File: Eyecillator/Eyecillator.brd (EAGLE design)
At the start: 92.4 x 35.5 mm, 24 parts, among them IC1 4093, IC2 LM567

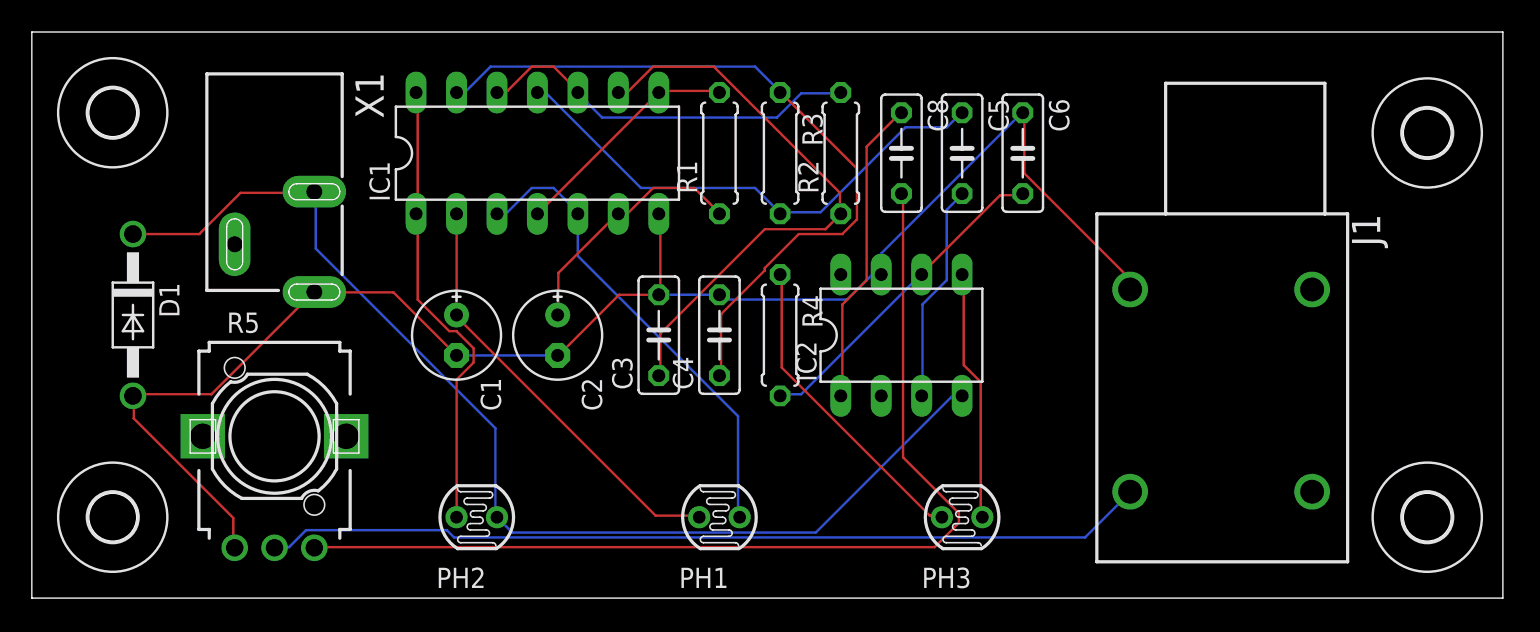
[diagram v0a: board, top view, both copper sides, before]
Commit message: Add files via upload
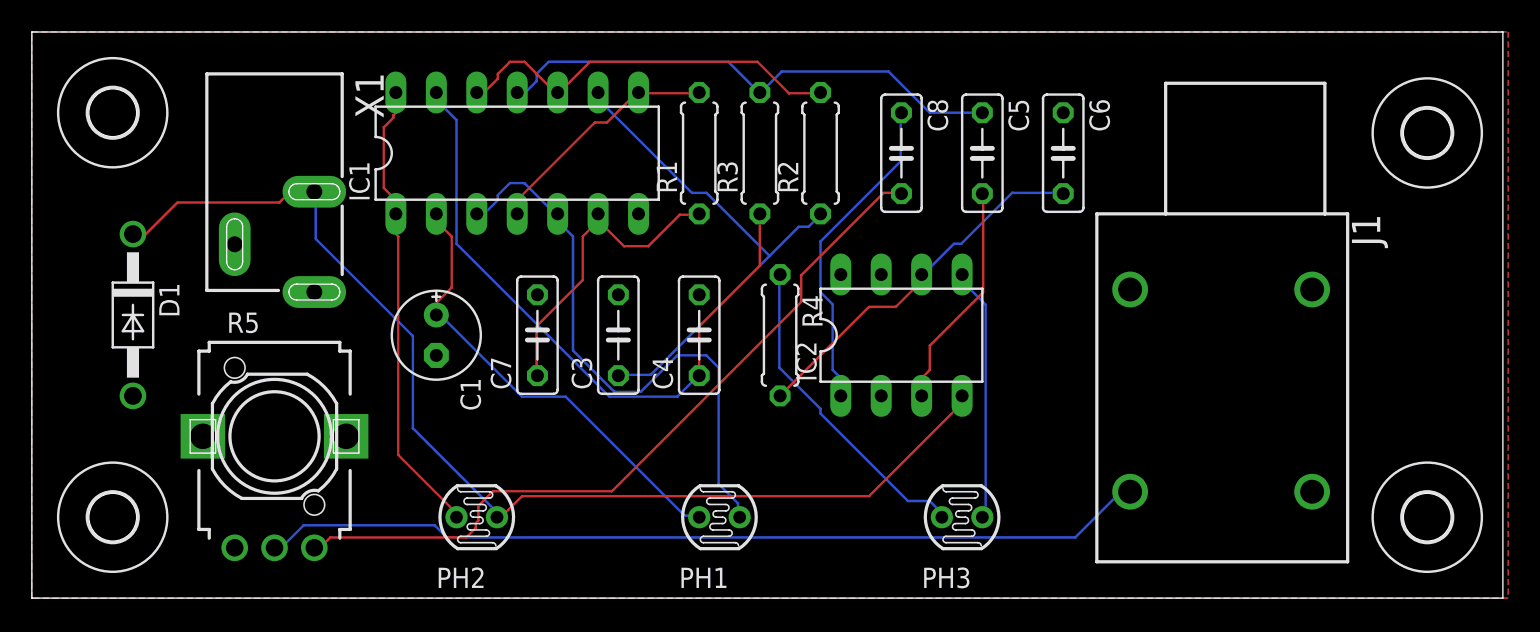
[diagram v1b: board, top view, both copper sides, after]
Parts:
- removed C2: 10uf, rcl:E2,5-6E
- added C7: 10uf, rcl:C050-025X075
- C4, C6, C8: value .1uf -> 0.1uf
- C5: value (none) -> 0.1uf
- moved C3 2.54 mm to (36.8, 16.5)
- moved C6 2.54 mm to (64.8, 27.9)
- moved C1 1.27 mm to (25.4, 16.5)
- moved C4 1.27 mm to (41.9, 16.5)
- moved R1 1.27 mm to (41.9, 27.9)
- moved R3 1.27 mm to (45.7, 27.9), turned to 90 degrees
- moved IC1 1.27 mm to (30.5, 27.9)
- moved C5 1.27 mm to (59.7, 27.9)
- moved R2 1.27 mm to (49.5, 27.9)
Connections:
- net GND: now also C7.2; no longer C2.-
- net N$5: now also C7.1; no longer C2.+
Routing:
- net GND: track 99.1 -> 0.00 mm
- net N$16: track 63.3 -> 47.8 mm
- net N$1: track 29.8 -> 37.3 mm
- net N$7: track 46.8 -> 41.6 mm
- net N$5: track 15.7 -> 20.1 mm
- net N$6: track 36.4 -> 32.2 mm
- net N$12: track 20.5 -> 23.4 mm
- net N$4: track 27.0 -> 29.0 mm
- net N$15: track 19.4 -> 20.4 mm
- net N$3: track 24.5 -> 25.1 mm
- net N$2: track 14.7 -> 15.3 mm
- net N$11: track 13.7 -> 14.3 mm
- net N$18: track 70.9 -> 70.3 mm
- added copper zone on layer 1, net GND
- added copper zone on layer 16, net GND
